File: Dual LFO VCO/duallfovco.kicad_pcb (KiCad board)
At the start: 2 copper layers, 40.3 x 128.5 mm, 17 parts

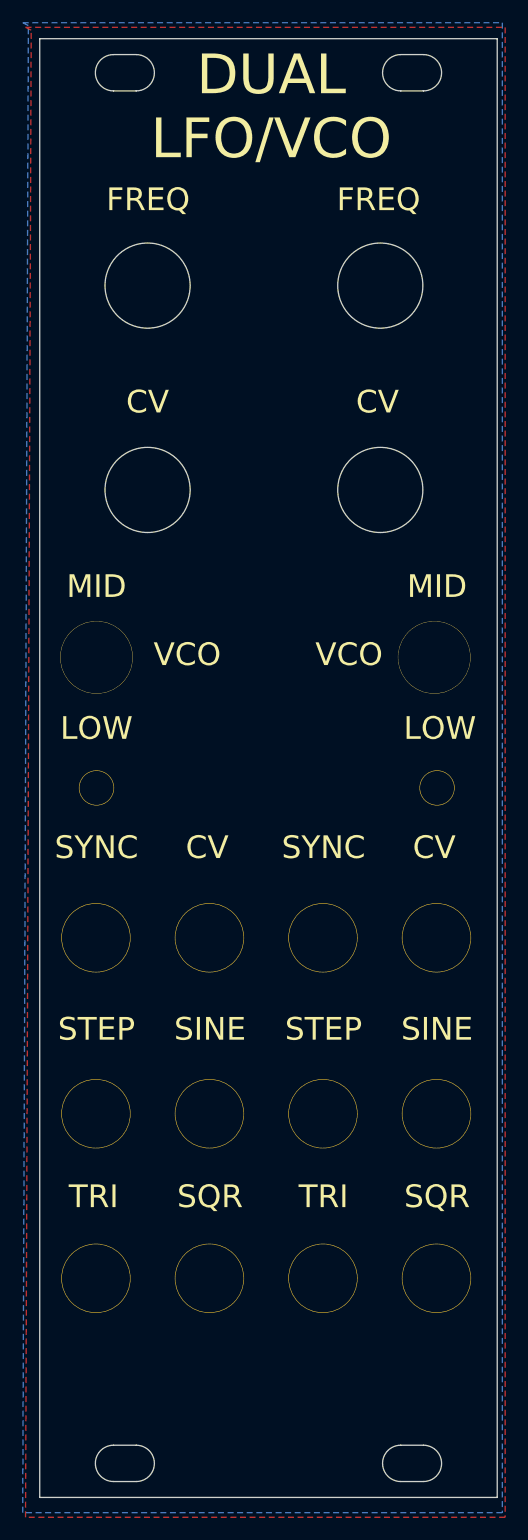
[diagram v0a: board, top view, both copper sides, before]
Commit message: Add files via upload
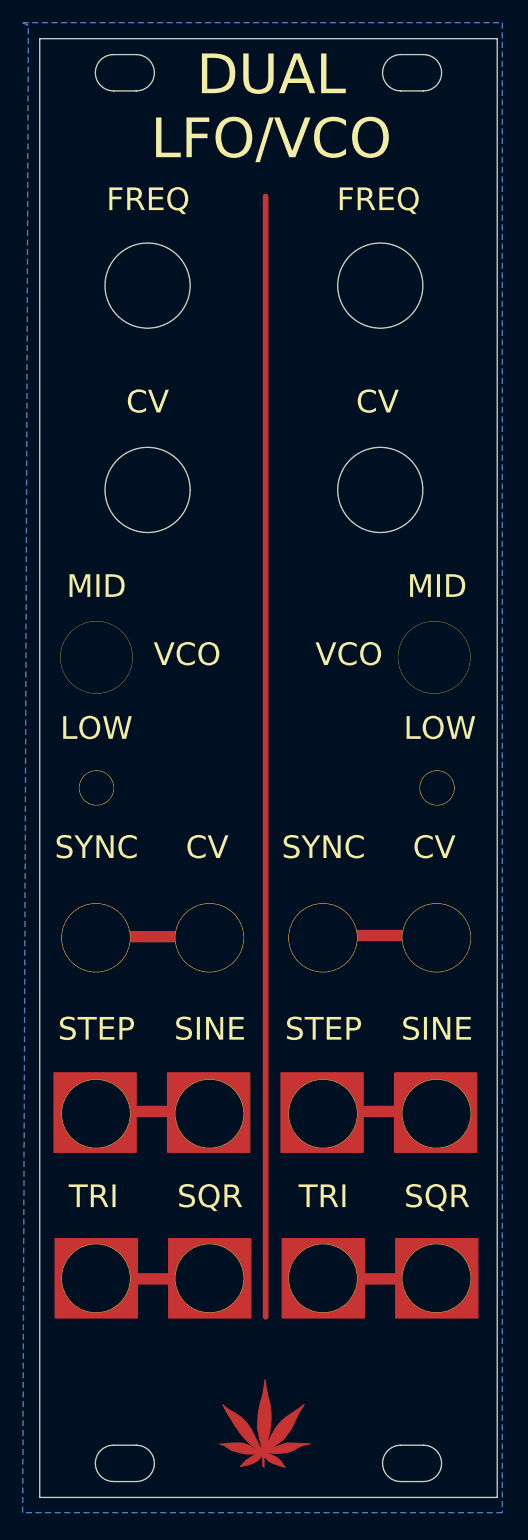
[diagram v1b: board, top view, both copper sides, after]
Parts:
- removed the REF** at (20.8, 121.5)
- added REF**: potleaf_small_copper, custom footprints:potleaf_small_copper, F.Cu at (19.8, 124.5)
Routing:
- removed copper zone on F.Cu, net GND
